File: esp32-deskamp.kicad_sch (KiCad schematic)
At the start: 3 parts, among them K1 TQ2-12V, U1 ESP32 D1 Mini, U2 TSR 1-2433

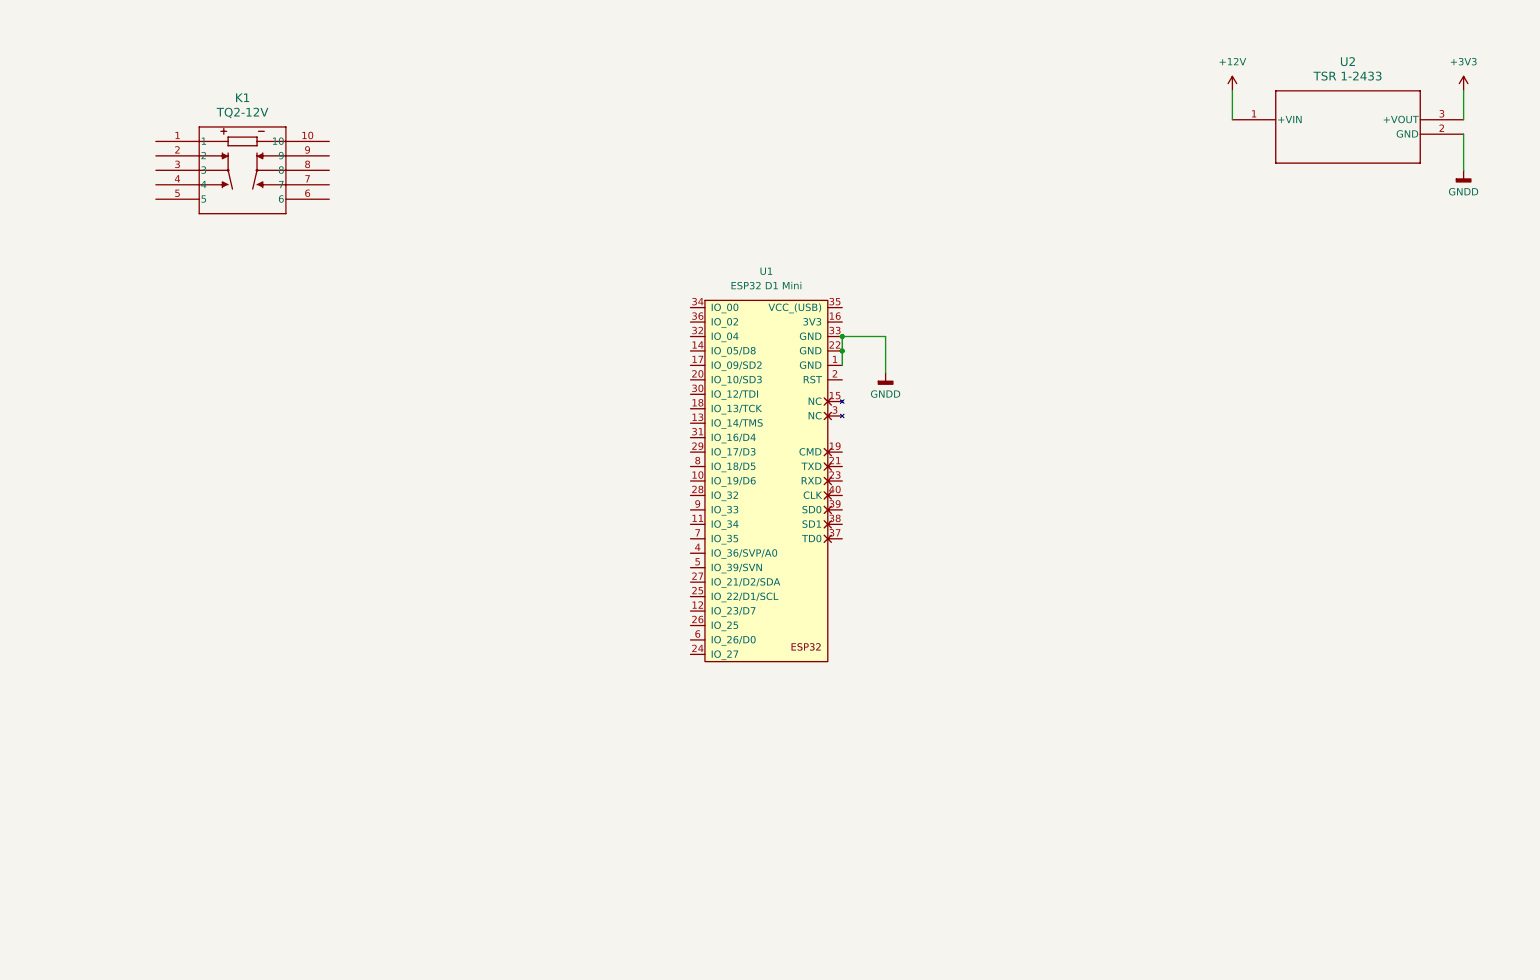
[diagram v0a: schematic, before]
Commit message: Rebuild chunk of schematic
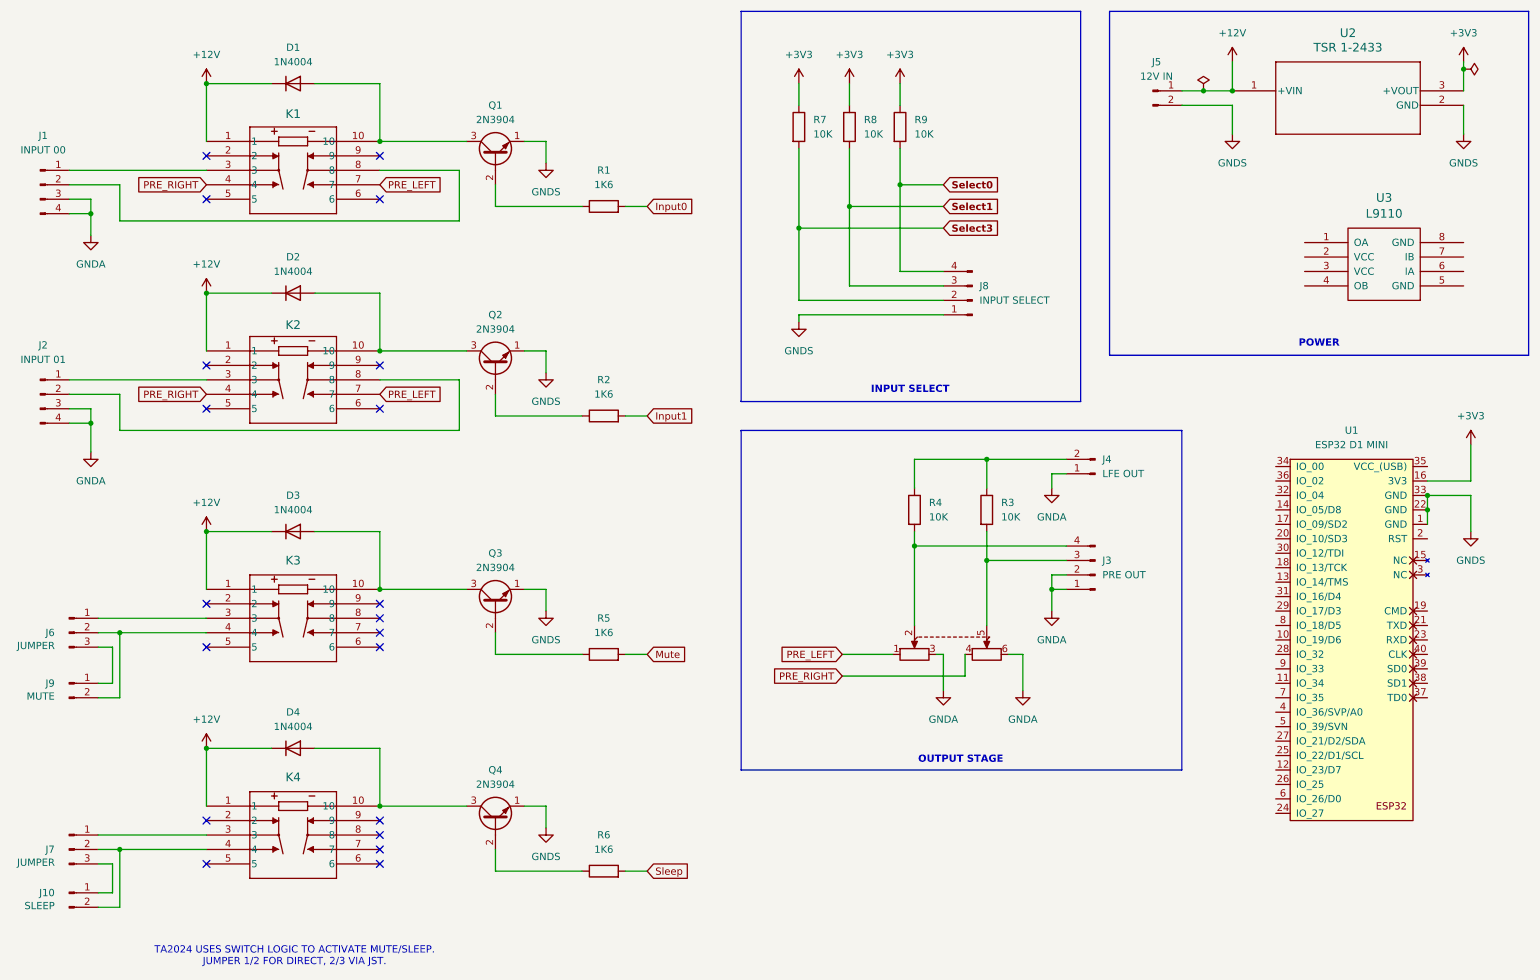
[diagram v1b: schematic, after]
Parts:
- added D1, D2, D3, D4: 1N4004, Diode_THT:D_DO-41_SOD81_P10.16mm_Horizontal, symbol Diode:1N4004
- added J1: INPUT 00, symbol Connector:Conn_01x04_Pin
- added J10: SLEEP, symbol Connector:Conn_01x02_Pin
- added J2: INPUT 01, symbol Connector:Conn_01x04_Pin
- added J3: PRE OUT, symbol Connector:Conn_01x04_Pin
- added J4: LFE OUT, symbol Connector:Conn_01x02_Pin
- added J5: 12V IN, symbol Connector:Conn_01x02_Pin
- added J6, J7: JUMPER, symbol Connector:Conn_01x03_Pin
- added J8: INPUT SELECT, symbol Connector:Conn_01x04_Pin
- added J9: MUTE, symbol Connector:Conn_01x02_Pin
- added K2: INPUT 01, RELAY_TQ2_PAN, symbol panasonic-tq2:TQ2-12V
- added K3: AMP MUTE, RELAY_TQ2_PAN, symbol panasonic-tq2:TQ2-12V
- added K4: AMP SLEEP, RELAY_TQ2_PAN, symbol panasonic-tq2:TQ2-12V
- added Q1, Q2, Q3, Q4: 2N3904, Package_TO_SOT_THT:TO-92_Inline, symbol Transistor_BJT:2N3904
- added R1, R2, R5, R6: 1K6, symbol Device:R
- added R3, R4, R7, R8, R9: 10K, symbol Device:R
- added RV1: RK27112MC, Potentiometer_THT:Potentiometer_Alps_RK27112MC, symbol custom:RK27112MC
- added U3: L9110, symbol L9110:L9110
- K1: value TQ2-12V -> INPUT 00
- U1: value ESP32 D1 Mini -> ESP32 D1 MINI
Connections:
- net +12V: now also K1.1, D1.1 (K), D2.1 (K), D3.1 (K), D4.1 (K), J5.1 (Pin_1), K2.1, K3.1, K4.1
- net +3V3: now also U1.16 (3V3), R7.1, R8.1, R9.1
- net at K1.10: now also D1.2 (A), Q1.3 (C)
- net at K1.3: now also J1.1 (Pin_1)
- net PRE_RIGHT: now reaches K1.4
- net PRE_RIGHT: now also K2.4, RV1.4
- net PRE_LEFT: now reaches K1.7
- net PRE_LEFT: now also K2.7, RV1.1
- net at K1.8: now also J1.2 (Pin_2)
- net GNDD renamed GNDS
- net GNDS: now also J5.2 (Pin_2), J8.1 (Pin_1), Q1.1 (E), Q2.1 (E), Q3.1 (E), Q4.1 (E)
- new net: Q1.2 (B), R1.1
- new net: Q4.2 (B), R6.1
- new net: D4.2 (A), K4.10, Q4.3 (C)
- new net: D3.2 (A), K3.10, Q3.3 (C)
- new net: J6.3 (Pin_3), J9.1 (Pin_1)
- new net: J6.2 (Pin_2), J9.2 (Pin_2), K3.4
- new net: J2.1 (Pin_1), K2.3
- new net: J2.2 (Pin_2), K2.8
- new net: D2.2 (A), K2.10, Q2.3 (C)
- new net: Q3.2 (B), R5.1
- new net: J10.1 (Pin_1), J7.3 (Pin_3)
- new net: J10.2 (Pin_2), J7.2 (Pin_2), K4.4
- new net: J4.2 (Pin_2), R3.1, R4.1
- new net: J3.3 (Pin_3), R3.2, RV1.5
- new net: J3.4 (Pin_4), R4.2, RV1.2
- new net: Q2.2 (B), R2.1
- new net: J7.1 (Pin_1), K4.3
- new net: J6.1 (Pin_1), K3.3
- new net GNDA: J1.3 (Pin_3), J1.4 (Pin_4), J2.3 (Pin_3), J2.4 (Pin_4), J3.1 (Pin_1), J3.2 (Pin_2), J4.1 (Pin_1), RV1.3, RV1.6
- new net Input0: R1.2
- new net Input1: R2.2
- new net Mute: R5.2
- new net Select0: J8.4 (Pin_4), R9.2
- new net Select1: J8.3 (Pin_3), R8.2
- new net Select3: J8.2 (Pin_2), R7.2
- new net Sleep: R6.2
- no-connect marks 0 -> 20
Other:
- note added: "INPUT SELECT"
- note added: "OUTPUT STAGE"
- note added: "POWER"
- note added: "TA2024 USES SWITCH LOGIC TO ACTIVATE MUTE/SLEEP. JUMPER 1/2 FOR DIRECT, 2/3 VIA JST."
- moved on the sheet: K1, U1, U2
